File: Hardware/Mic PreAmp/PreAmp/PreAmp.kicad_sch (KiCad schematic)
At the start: 7 parts, among them J1 Conn_01x05_Pin, J2 Conn_01x03_Pin, J3 XLR3, U1 TLV2371DBV, U2 INA217AIDWR

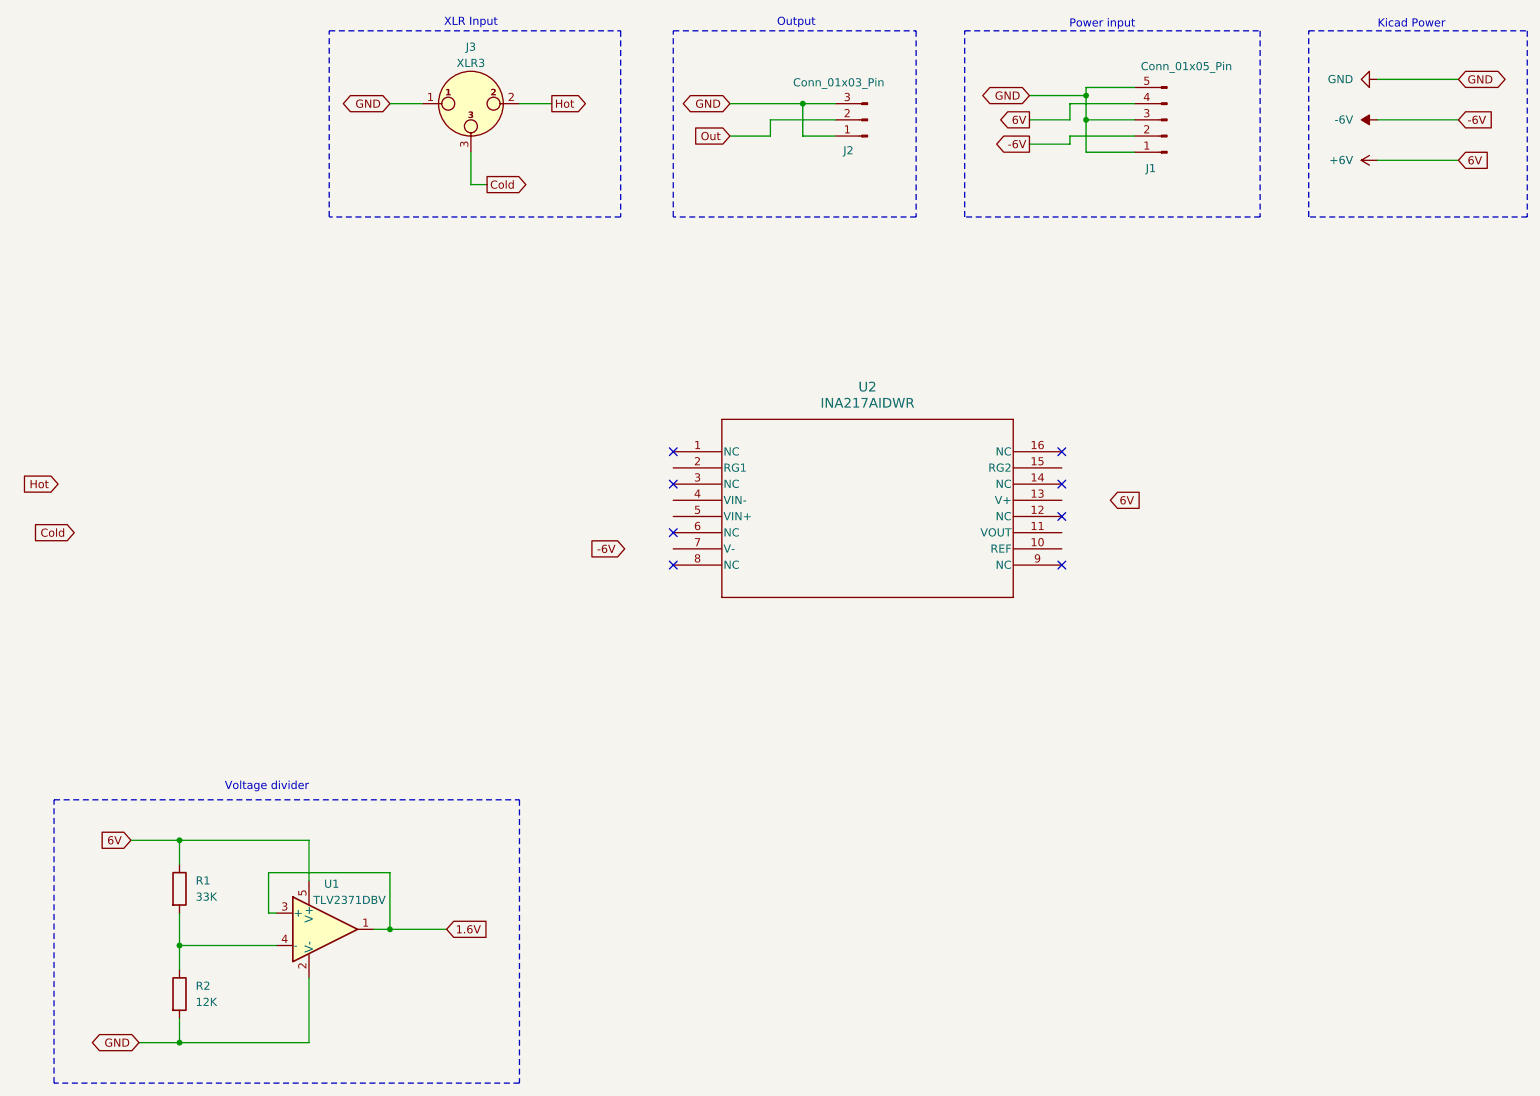
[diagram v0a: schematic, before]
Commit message: Circuit before V_In
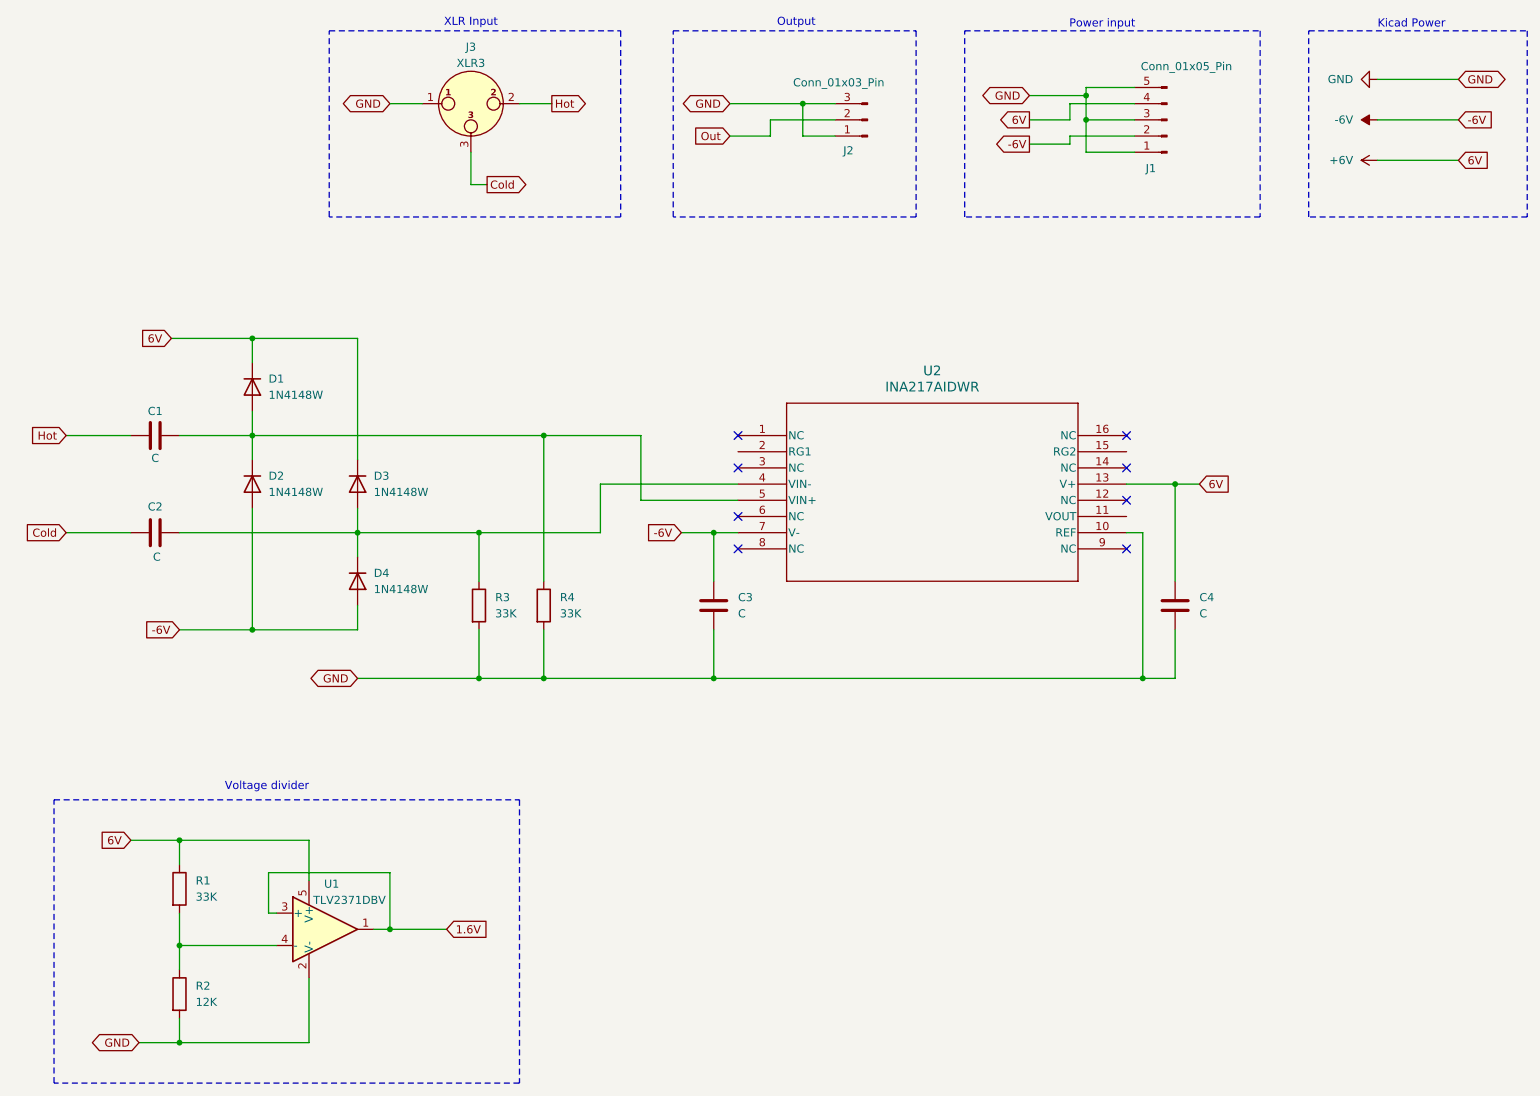
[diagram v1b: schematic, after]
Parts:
- added C1, C2, C3, C4: C, symbol Device:C
- added D1, D2, D3, D4: 1N4148W, Diode_THT:D_DO-35_SOD27_P7.62mm_Horizontal, symbol Diode:1N4148W
- added R3, R4: 33K, symbol Device:R
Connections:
- net +6V: now also U2.13 (V+), C4.1, D1.1 (K), D3.1 (K)
- net -6V: now also U2.7 (V-), C3.1, D2.2 (A), D4.2 (A)
- net Cold: now also C2.1
- net GND: now also U2.10 (REF), C3.2, C4.2, R3.2, R4.2
- net Hot: now also C1.1
- net at U2.4 (VIN-): now also C2.2, D3.2 (A), D4.1 (K), R3.1
- net at U2.5 (VIN+): now also C1.2, D1.2 (A), D2.1 (K), R4.1
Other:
- moved on the sheet: U2
